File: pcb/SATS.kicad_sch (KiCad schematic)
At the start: 13 parts, among them J1 Raspberry_Pi_2_3, SW1 SW_Reed, SW2 SW_Reed, SW3 SW_Reed, U1 MCP23017_SP, U2 MCP23017_SP, U3 CD40109BE, U4 IRLZ14PBF

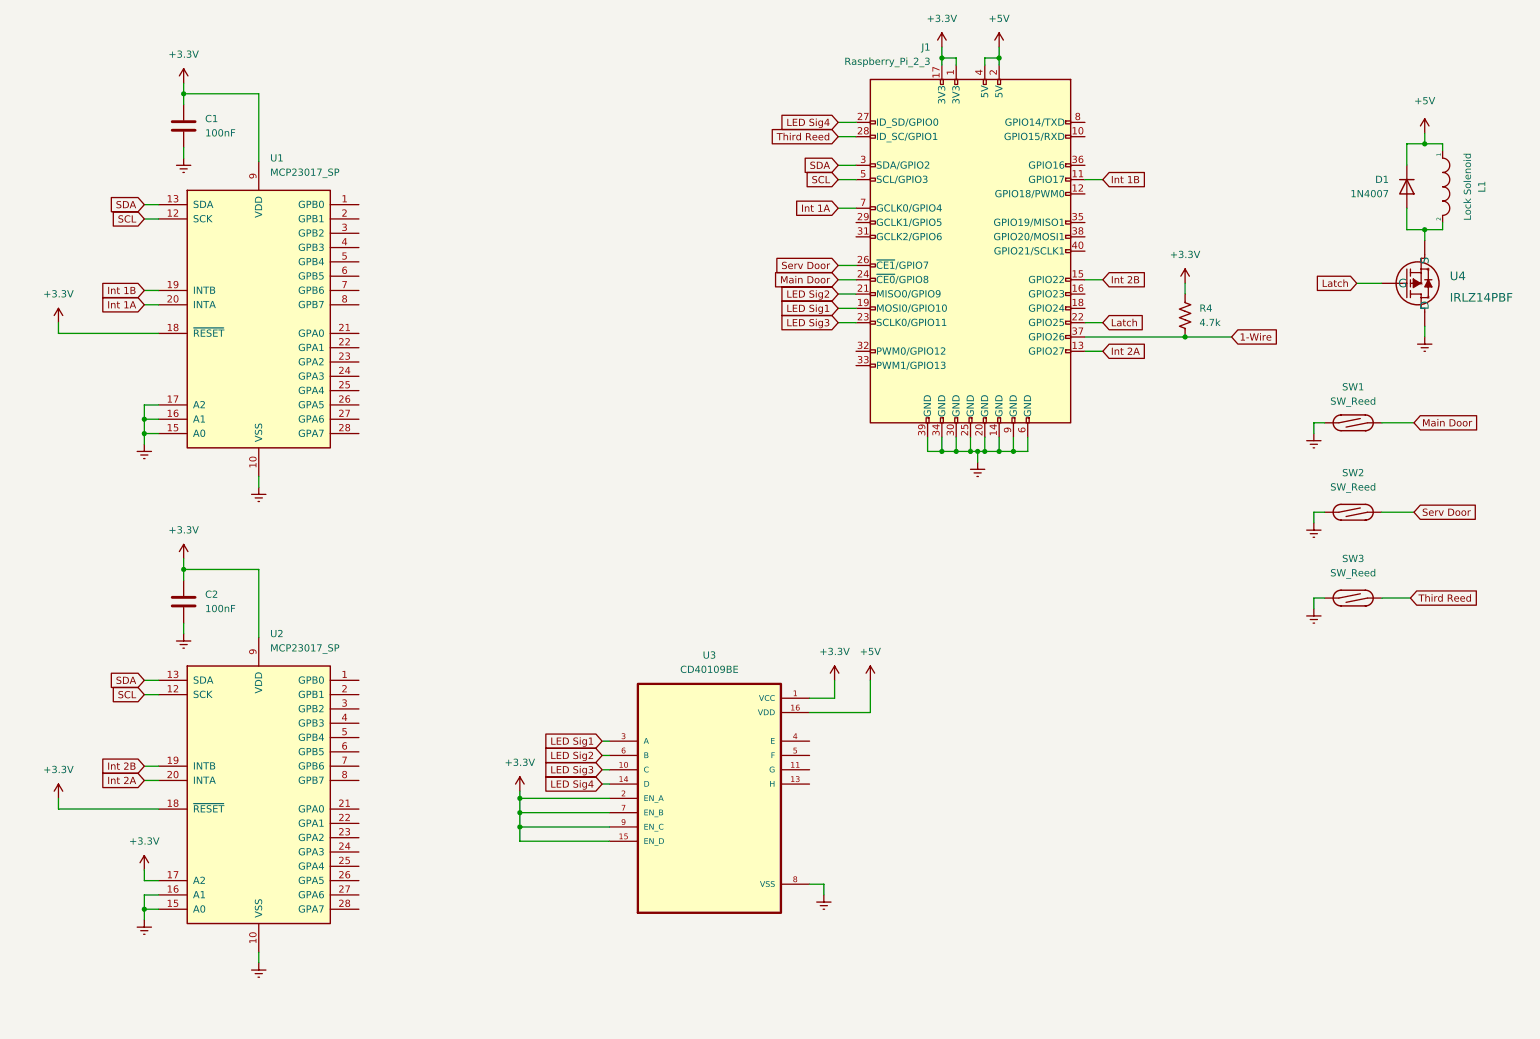
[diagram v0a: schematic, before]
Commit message: Route jacks
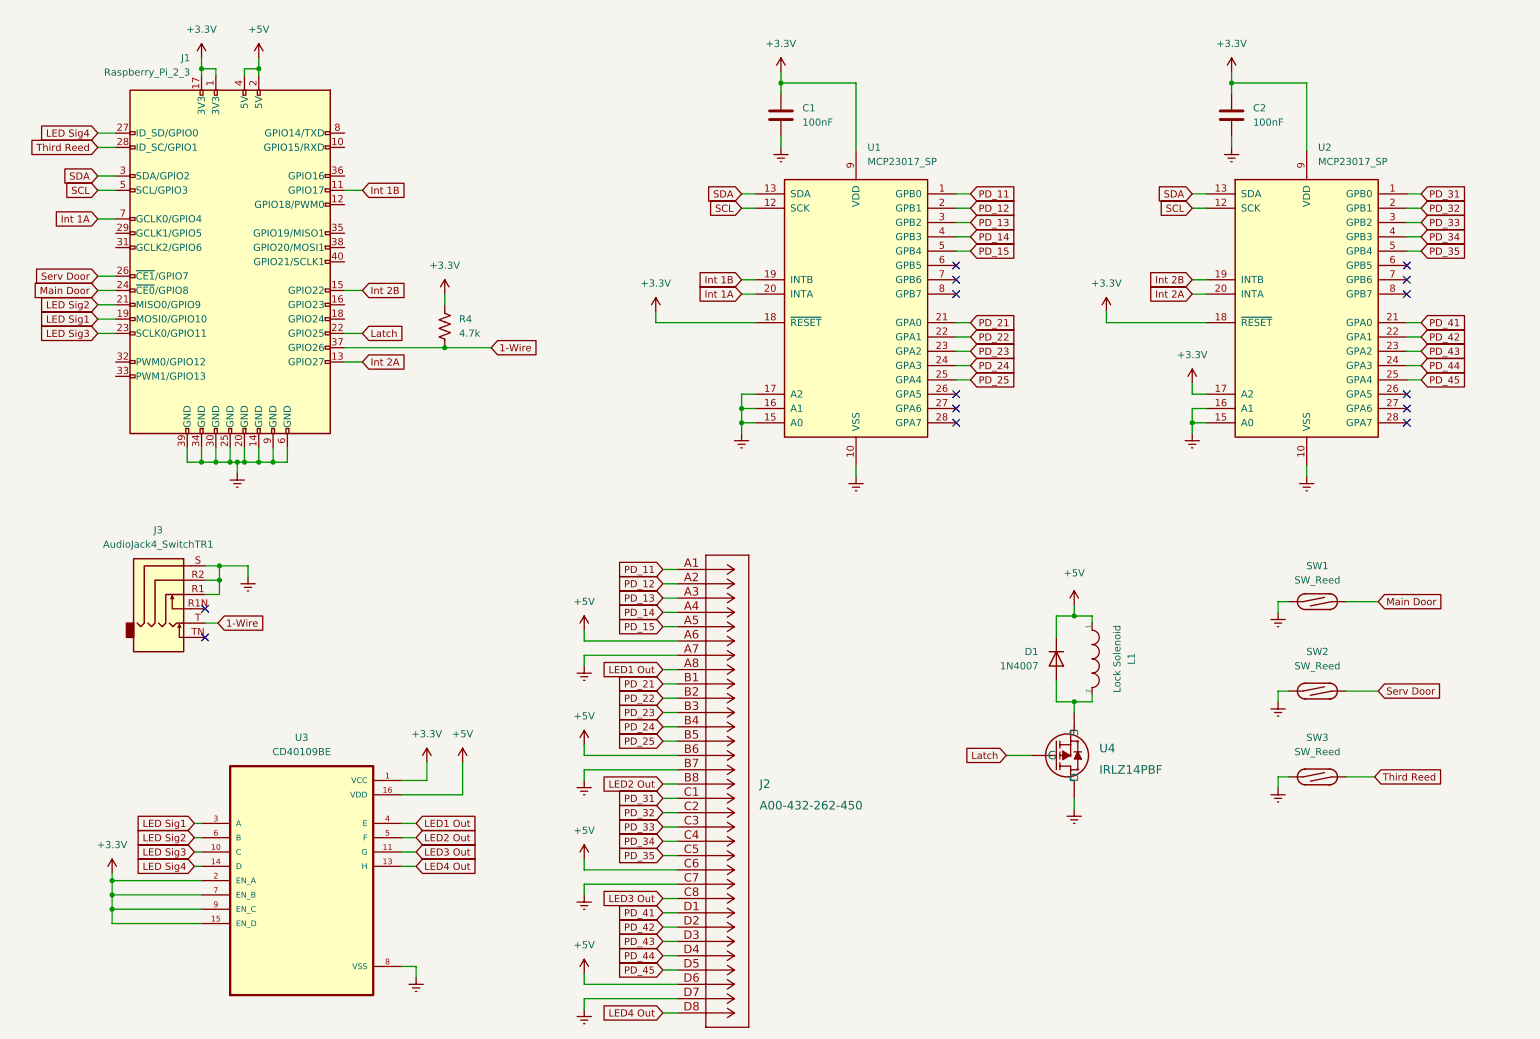
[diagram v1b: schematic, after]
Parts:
- added J2: A00-432-262-450, CONN_A00-432-262-450_EDA, symbol QuadRJ45:A00-432-262-450
- added J3: AudioJack4_SwitchTR1, symbol Connector:AudioJack4_SwitchTR1
- C1, C2: footprint (none) -> Capacitor_THT:C_Rect_L7.0mm_W3.5mm_P5.00mm
- R4: footprint (none) -> Resistor_THT:R_Axial_DIN0207_L6.3mm_D2.5mm_P7.62mm_Horizontal
- U3: footprint DIP794W45P254L1969H508Q16 -> CD40109BE:DIP794W45P254L1969H508Q16
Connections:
- net +5V: now also J2.A6, J2.B6, J2.C6, J2.D6
- net 1-Wire: now also J3.T
- net Earth: now also J2.A7, J2.B7, J2.C7, J2.D7, J3.R1, J3.R2, J3.S
- net LED3 Out: now reaches U3.11 (G)
- net LED3 Out: now also J2.C8
- net LED4 Out: now reaches U3.13 (H)
- net LED4 Out: now also J2.D8
- net LED1 Out: now reaches U3.4 (E)
- net LED1 Out: now also J2.A8
- net LED2 Out: now reaches U3.5 (F)
- net LED2 Out: now also J2.B8
- net PD_11: now reaches U1.1 (GPB0)
- net PD_11: now also J2.A1
- net PD_12: now reaches U1.2 (GPB1)
- net PD_12: now also J2.A2
- net PD_21: now reaches U1.21 (GPA0)
- net PD_21: now also J2.B1
- net PD_22: now reaches U1.22 (GPA1)
- net PD_22: now also J2.B2
- net PD_23: now reaches U1.23 (GPA2)
- net PD_23: now also J2.B3
- net PD_24: now reaches U1.24 (GPA3)
- net PD_24: now also J2.B4
- net PD_25: now reaches U1.25 (GPA4)
- net PD_25: now also J2.B5
- net PD_13: now reaches U1.3 (GPB2)
- net PD_13: now also J2.A3
- net PD_14: now reaches U1.4 (GPB3)
- net PD_14: now also J2.A4
- net PD_15: now reaches U1.5 (GPB4)
- net PD_15: now also J2.A5
- net PD_31: now reaches U2.1 (GPB0)
- net PD_31: now also J2.C1
- net PD_32: now reaches U2.2 (GPB1)
- net PD_32: now also J2.C2
- net PD_41: now reaches U2.21 (GPA0)
- net PD_41: now also J2.D1
- net PD_42: now reaches U2.22 (GPA1)
- net PD_42: now also J2.D2
- net PD_43: now reaches U2.23 (GPA2)
- net PD_43: now also J2.D3
- net PD_44: now reaches U2.24 (GPA3)
- net PD_44: now also J2.D4
- net PD_45: now reaches U2.25 (GPA4)
- net PD_45: now also J2.D5
- net PD_33: now reaches U2.3 (GPB2)
- net PD_33: now also J2.C3
- net PD_34: now reaches U2.4 (GPB3)
- net PD_34: now also J2.C4
- net PD_35: now reaches U2.5 (GPB4)
- net PD_35: now also J2.C5
- no-connect marks 0 -> 14
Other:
- moved on the sheet: C1, C2, D1, J1, L1, R4, SW1, SW2, SW3, U1, U2, U3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
